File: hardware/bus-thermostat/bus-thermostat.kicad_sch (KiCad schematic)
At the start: 0 parts

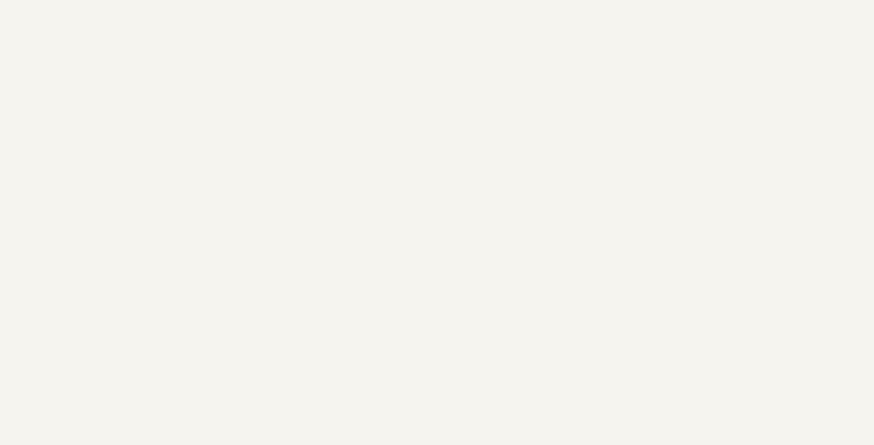
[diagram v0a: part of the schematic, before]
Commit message: First rev of thermostat firmware
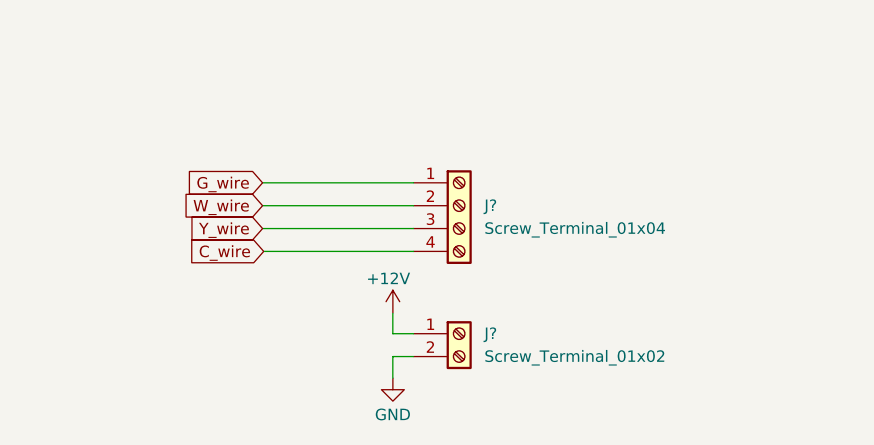
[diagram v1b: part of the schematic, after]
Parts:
- added J?: Screw_Terminal_01x02, symbol Connector:Screw_Terminal_01x02
- added J?: Screw_Terminal_01x04, symbol Connector:Screw_Terminal_01x04
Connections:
- new net +12V: J?.1 (Pin_1)
- new net C_wire: J?.4 (Pin_4)
- new net GND: J?.2 (Pin_2)
- new net G_wire: J?.1 (Pin_1)
- new net W_wire: J?.2 (Pin_2)
- new net Y_wire: J?.3 (Pin_3)
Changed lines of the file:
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@@
 (kicad_sch (version 20211123) (generator eeschema)
   (paper "A4")
+  (wire (pts (xy 49.022 101.473) (xy 65.786 101.473))
+    (stroke (width 0) (type default) (color 0 0 0 0))
+  )
+  (wire (pts (xy 65.786 113.157) (xy 63.5 113.157))
+    (stroke (width 0) (type default) (color 0 0 0 0))
+  )
+  (wire (pts (xy 49.022 98.933) (xy 65.786 98.933))
+    (stroke (width 0) (type default) (color 0 0 0 0))
+  )
+  (wire (pts (xy 63.5 115.697) (xy 65.786 115.697))
+    (stroke (width 0) (type default) (color 0 0 0 0))
+  )
+  (wire (pts (xy 49.022 96.393) (xy 65.786 96.393))
+    (stroke (width 0) (type default) (color 0 0 0 0))
+  )
+  (wire (pts (xy 63.5 110.871) (xy 63.5 113.157))
+    (stroke (width 0) (type default) (color 0 0 0 0))
+  )
+  (wire (pts (xy 63.5 118.11) (xy 63.5 115.697))
+    (stroke (width 0) (type default) (color 0 0 0 0))
+  )
+  (wire (pts (xy 49.149 104.013) (xy 65.786 104.013))
+    (stroke (width 0) (type default) (color 0 0 0 0))
+  )
+  (global_label "Y_wire" (shape input) (at 49.022 101.473 180) (fields_autoplaced)
+    (effects (font (size 1.27 1.27)) (justify right))
+    (property "Intersheet References" "${INTERSHEET_REFS}" (id 0) (at 40.7427 101.3936 0)
+      (effects (font (size 1.27 1.27)) (justify right) hide)
+    )
+  )
+  (global_label "W_wire" (shape input) (at 49.022 98.933 180) (fields_autoplaced)
+    (effects (font (size 1.27 1.27)) (justify right))
+    (property "Intersheet References" "${INTERSHEET_REFS}" (id 0) (at 40.3799 98.8536 0)
+      (effects (font (size 1.27 1.27)) (justify right) hide)
+    )
+  )
+  (global_label "C_wire" (shape input) (at 49.149 104.013 180) (fields_autoplaced)
+    (effects (font (size 1.27 1.27)) (justify right))
+    (property "Intersheet References" "${INTERSHEET_REFS}" (id 0) (at 40.6883 103.9336 0)
+      (effects (font (size 1.27 1.27)) (justify right) hide)
+    )
+  )
+  (global_label "G_wire" (shape input) (at 49.022 96.393 180) (fields_autoplaced)
+    (effects (font (size 1.27 1.27)) (justify right))
+    (property "Intersheet References" "${INTERSHEET_REFS}" (id 0) (at 40.5613 96.3136 0)
+      (effects (font (size 1.27 1.27)) (justify right) hide)
+    )
+  )
+  (symbol (lib_id "power:+12V") (at 63.5 110.871 0) (unit 1)
+    (in_bom yes) (on_board yes)
+    (property "Reference" "#PWR?" (id 0) (at 63.5 114.681 0)
+      (effects (font (size 1.27 1.27)) hide)
+    )
+    (property "Value" "+12V" (id 1) (at 62.992 107.061 0))
+    (property "Footprint" "" (id 2) (at 63.5 110.871 0)
+      (effects (font (size 1.27 1.27)) hide)
+    )
+    (property "Datasheet" "" (id 3) (at 63.5 110.871 0)
+      (effects (font (size 1.27 1.27)) hide)
+    )
+    (pin "1")
+  )
+  (symbol (lib_id "Connector:Screw_Terminal_01x02") (at 70.866 113.157 0) (unit 1)
+    (in_bom yes) (on_board yes) (fields_autoplaced)
+    (property "Reference" "J?" (id 0) (at 73.66 113.1569 0)
+      (effects (font (size 1.27 1.27)) (justify left))
+    )
+    (property "Value" "Screw_Terminal_01x02" (id 1) (at 73.66 115.6969 0)
+      (effects (font (size 1.27 1.27)) (justify left))
+    )
+    (property "Footprint" "" (id 2) (at 70.866 113.157 0)
+      (effects (font (size 1.27 1.27)) hide)
+    )
+    (property "Datasheet" "~" (id 3) (at 70.866 113.157 0)
+      (effects (font (size 1.27 1.27)) hide)
+    )
+    (pin "1")
+    (pin "2")
+  )
+  (symbol (lib_id "power:GND") (at 63.5 118.11 0) (unit 1)
+    (in_bom yes) (on_board yes)
+    (property "Reference" "#PWR?" (id 0) (at 63.5 124.46 0)
+      (effects (font (size 1.27 1.27)) hide)
+    )
+    (property "Value" "GND" (id 1) (at 63.5 122.174 0))
+    (property "Footprint" "" (id 2) (at 63.5 118.11 0)
+      (effects (font (size 1.27 1.27)) hide)
+    )
+    (property "Datasheet" "" (id 3) (at 63.5 118.11 0)
+      (effects (font (size 1.27 1.27)) hide)
+    )
+    (pin "1")
+  )
+  (symbol (lib_id "Connector:Screw_Terminal_01x04") (at 70.866 98.933 0) (unit 1)
+    (in_bom yes) (on_board yes) (fields_autoplaced)
+    (property "Reference" "J?" (id 0) (at 73.66 98.9329 0)
+      (effects (font (size 1.27 1.27)) (justify left))
+    )
+    (property "Value" "Screw_Terminal_01x04" (id 1) (at 73.66 101.4729 0)
+      (effects (font (size 1.27 1.27)) (justify left))
+    )
+    (property "Footprint" "" (id 2) (at 70.866 98.933 0)
+      (effects (font (size 1.27 1.27)) hide)
+    )
+    (property "Datasheet" "~" (id 3) (at 70.866 98.933 0)
+      (effects (font (size 1.27 1.27)) hide)
+    )
+    (pin "1")
+    (pin "2")
+    (pin "3")
+    (pin "4")
+  )
   (sheet (at 17.78 20.32) (size 55.88 34.29) (fields_autoplaced)
     (stroke (width 0.1524) (type solid) (color 0 0 0 0))
@@
       (reference "#PWR060") (unit 1) (value "GND") (footprint "")
     )
-    (path "/9a2fdddb-dad5-445e-a65c-2bfabfe3e5b9/95c2153b-4868-4c8f-873d-3268ea7ecfa7"
-      (reference "#PWR061") (unit 1) (value "+3V3") (footprint "")
-    )
-    (path "/9a2fdddb-dad5-445e-a65c-2bfabfe3e5b9/7ff05544-1504-476a-b892-5f01c5e034c4"
-      (reference "#PWR062") (unit 1) (value "GND") (footprint "")
-    )
     (path "/9a2fdddb-dad5-445e-a65c-2bfabfe3e5b9/a5f099e4-c633-414a-9719-1483d3540102"
       (reference "#PWR063") (unit 1) (value "GND") (footprint "")
@@
       (reference "#PWR0101") (unit 1) (value "-6V") (footprint "")
     )
+    (path "/e9a8718b-cce8-4a1a-9229-65779783a760/19e5e61e-4904-4fc2-a889-225a6f9529ad"
+      (reference "#PWR?") (unit 1) (value "GND") (footprint "")
+    )
+    (path "/2295b6ba-5c88-4e72-82fd-1de2cde8ad5c"
+      (reference "#PWR?") (unit 1) (value "+12V") (footprint "")
+    )
+    (path "/5225554a-3241-4eb4-9fd0-3f5061d0114a/2fb33cd7-f53e-4e9a-b1b4-f762c80e1ceb"
+      (reference "#PWR?") (unit 1) (value "GND") (footprint "")
+    )
+    (path "/5e83791a-22fa-4ad9-b200-df9a0fa51bd9"
+      (reference "#PWR?") (unit 1) (value "GND") (footprint "")
+    )
+    (path "/5225554a-3241-4eb4-9fd0-3f5061d0114a/8e31a8b0-9b04-4808-b7db-b4ea38283047"
+      (reference "#PWR?") (unit 1) (value "GND") (footprint "")
+    )
+    (path "/9a2fdddb-dad5-445e-a65c-2bfabfe3e5b9/9fe15f6f-8a99-4fe5-b2cb-39ca50568b71"
+      (reference "#PWR?") (unit 1) (value "+3V3") (footprint "")
+    )
+    (path "/9a2fdddb-dad5-445e-a65c-2bfabfe3e5b9/c767a628-9ce5-4e99-b0d6-9ffd51f2e266"
+      (reference "#PWR?") (unit 1) (value "GND") (footprint "")
+    )
+    (path "/5225554a-3241-4eb4-9fd0-3f5061d0114a/d0c84035-13b5-4e42-a768-c225322551a3"
+      (reference "#PWR?") (unit 1) (value "+3V3") (footprint "")
+    )
     (path "/5225554a-3241-4eb4-9fd0-3f5061d0114a/5416d296-3963-4899-9169-65cf2055b600"
       (reference "C1") (unit 1) (value "220pF") (footprint "")
@@
       (reference "C37") (unit 1) (value "100nF") (footprint "")
     )
+    (path "/b3446cb0-6e23-490d-8c96-4b8b72cbbdab/d8843b58-d803-4641-9b81-1964b29aca15"
+      (reference "C?") (unit 1) (value "470nF") (footprint "")
+    )
     (path "/5225554a-3241-4eb4-9fd0-3f5061d0114a/9921d59a-479e-4581-9892-34f37467aa18"
       (reference "D1") (unit 1) (value "LMB14S") (footprint "Diode_SMD:Diode_Bridge_Vishay_MBLS")
@@
       (reference "D12") (unit 1) (value "BAT54J") (footprint "Diode_SMD:D_SOD-323F")
     )
-    (path "/9a2fdddb-dad5-445e-a65c-2bfabfe3e5b9/a3d1acdc-5d8c-4ff6-8dae-71a976d7c1fc"
-      (reference "J1") (unit 1) (value "Conn_01x03_Female") (footprint "")
+    (path "/9a2fdddb-dad5-445e-a65c-2bfabfe3e5b9/739ce458-cbf7-4287-8a10-b8dd4eb792fe"
+      (reference "D?") (unit 1) (value "BAT42W-V") (footprint "Diode_SMD:D_SOD-123")
+    )
+    (path "/e9a8718b-cce8-4a1a-9229-65779783a760/ac1e7681-48cb-4190-8867-f5ff3d478e49"
+      (reference "D?") (unit 1) (value "18V Zener") (footprint "")
     )
     (path "/9a2fdddb-dad5-445e-a65c-2bfabfe3e5b9/fedf54aa-e23c-4192-8197-589a4b54af2f"
       (reference "J2") (unit 1) (value "RJ45_Shielded") (footprint "")
     )
+    (path "/58693072-0665-4444-9819-189d4fe97e8f"
+      (reference "J?") (unit 1) (value "Screw_Terminal_01x02") (footprint "")
+    )
+    (path "/71a196c3-2ba1-4e87-8601-8cd342758170"
+      (reference "J?") (unit 1) (value "Screw_Terminal_01x04") (footprint "")
+    )
+    (path "/9a2fdddb-dad5-445e-a65c-2bfabfe3e5b9/ec66682e-00f4-44dc-9e5e-2b2cdb8a8a1f"
+      (reference "J?") (unit 1) (value "FTDI Serial") (footprint "SparkFun-Connectors:6_PIN_SERIAL_TARGET_SIDE_W_SILK")
+    )
+    (path "/9a2fdddb-dad5-445e-a65c-2bfabfe3e5b9/d131077e-2109-4a2c-85dc-1939ce9a83fe"
+      (reference "JP?") (unit 1) (value "Solder Jumper") (footprint "Jumper:SolderJumper-2_P1.3mm_Open_TrianglePad1.0x1.5mm")
+    )
     (path "/5225554a-3241-4eb4-9fd0-3f5061d0114a/b9509bd5-25af-4378-b6b0-d098fb79c657"
       (reference "L1") (unit 1) (value "100mH") (footprint "")
@@
       (reference "R46") (unit 1) (value "10k") (footprint "")
     )
+    (path "/9a2fdddb-dad5-445e-a65c-2bfabfe3e5b9/10990986-19d1-4e7a-87b5-88d2b2cd50b8"
+      (reference "R?") (unit 1) (value "470R") (footprint "")
+    )
+    (path "/5225554a-3241-4eb4-9fd0-3f5061d0114a/7e4d14b9-ef9a-4b98-af8f-b239a9ae5175"
+      (reference "R?") (unit 1) (value "10k") (footprint "")
+    )
+    (path "/5225554a-3241-4eb4-9fd0-3f5061d0114a/c372fdac-807e-4682-a91c-559f1b825eaa"
+      (reference "R?") (unit 1) (value "10k") (footprint "")
+    )
     (path "/b3446cb0-6e23-490d-8c96-4b8b72cbbdab/eeac21de-3d26-4236-8cca-48baa88e445a"
       (reference "RV1") (unit 1) (value "50k") (footprint "")
@@
       (reference "U14") (unit 1) (value "TLV9301IDCK") (footprint "Package_TO_SOT_SMD:SOT-353_SC-70-5")
     )
-  )
+    (path "/5225554a-3241-4eb4-9fd0-3f5061d0114a/0ba209e5-47d3-4e1d-b5c2-2758757a26c8"
+      (reference "U?") (unit 1) (value "PCA9557D") (footprint "Package_SO:SOP-16_3.9x9.9mm_P1.27mm")
+    )
+  )
